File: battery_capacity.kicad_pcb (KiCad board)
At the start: 2 copper layers, 47 x 45 mm, 17 parts, among them J1 Screw_Terminal_01x03, J2 Screw_Terminal_01x04, Q1 IRLML2060, Q2 IRLML2060, U1 PC817, U2 PC817, U3 YAAJ_DCDC_StepDown_LM2596

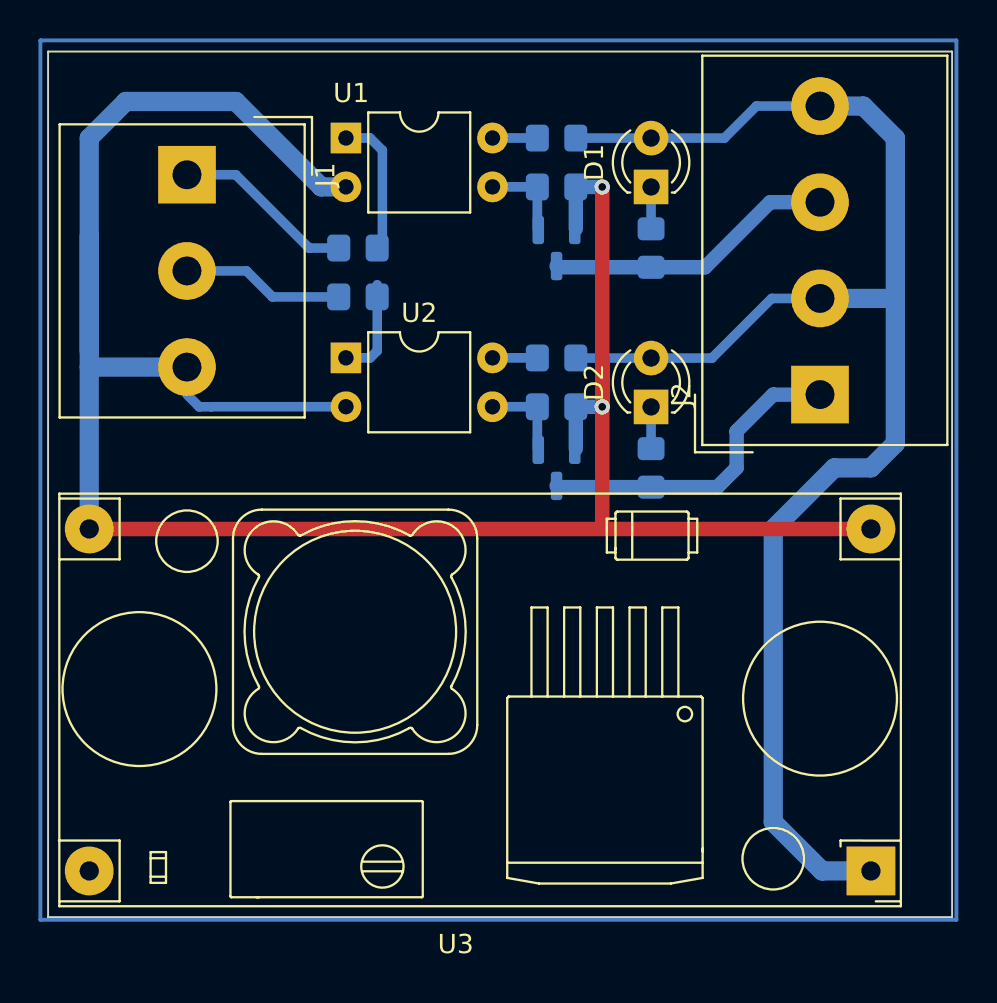
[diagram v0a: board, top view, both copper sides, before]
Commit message: h
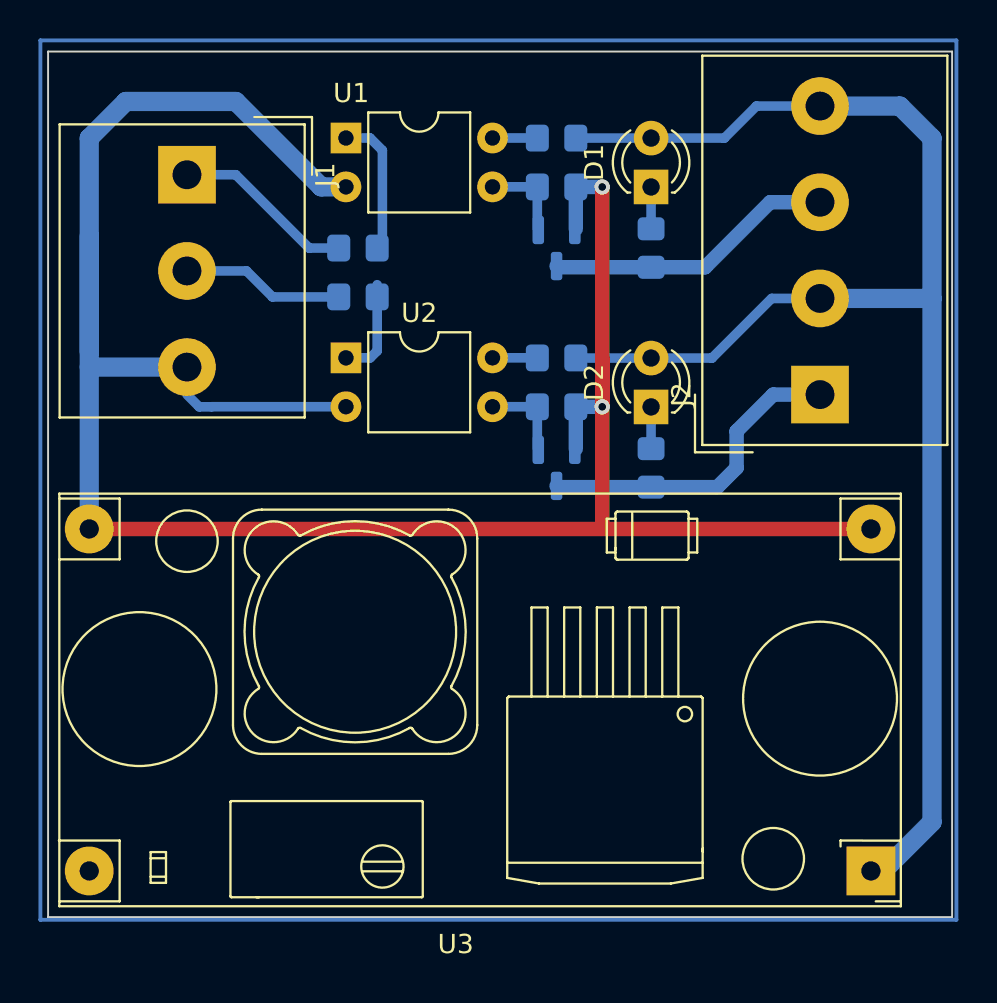
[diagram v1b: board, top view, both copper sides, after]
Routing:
- net +24V: track 81.4 -> 79.5 mm
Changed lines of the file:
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@@
     (fp_arc (start 9.481636 16.283217) (mid 9.510921 16.212508) (end 9.581636 16.183217)
       (stroke (width 0.12) (type solid)) (layer "F.SilkS"))
-    (fp_arc (start 9.581636 18.683217) (mid 9.510896 18.653941) (end 9.481636 18.583217)
-      (stroke (width 0.12) (type solid)) (layer "F.SilkS"))
-    (fp_arc (start 13.181636 16.183217) (mid 13.252317 16.21252) (end 13.281636 16.283217)
+    (fp_arc (start 9.581636 18.683217) (mid 9.510931 18.653935) (end 9.481636 18.583217)
+      (stroke (width 0.12) (type solid)) (layer "F.SilkS"))
+    (fp_arc (start 13.181636 16.183217) (mid 13.252353 16.212514) (end 13.281636 16.283217)
       (stroke (width 0.12) (type solid)) (layer "F.SilkS"))
     (fp_arc (start 13.281636 18.583217) (mid 13.252343 18.653929) (end 13.181636 18.683217)
@@
     (fp_arc (start 23.847611 17.472062) (mid 21.514153 17.739048) (end 21.781132 15.405582)
       (stroke (width 0.12) (type solid)) (layer "F.SilkS"))
-    (fp_arc (start 23.847611 17.472062) (mid 23.907831 17.428018) (end 23.981783 17.437976)
+    (fp_arc (start 23.847611 17.472062) (mid 23.907835 17.428062) (end 23.981783 17.437976)
       (stroke (width 0.12) (type solid)) (layer "F.SilkS"))
     (fp_arc (start 23.981783 7.433617) (mid 23.907854 7.443509) (end 23.847611 7.399531)
@@
     (stroke (width 0.1) (type default)) (fill none) (layer "Edge.Cuts"))
   (segment (start 133.35 68.215) (end 133.35 66.04) (width 0.5) (layer "B.Cu") (net 1))
-  (segment (start 146.05 63.5) (end 146.05 79.375) (width 1) (layer "B.Cu") (net 2))
-  (segment (start 146.05 79.375) (end 144.78 80.645) (width 1) (layer "B.Cu") (net 2))
-  (segment (start 145.97 71.835) (end 142.1325 71.835) (width 1) (layer "B.Cu") (net 2))
-  (segment (start 139.7 99.06) (end 142.24 101.6) (width 1) (layer "B.Cu") (net 2))
   (segment (start 129.435 74.93) (end 129.44 74.935) (width 0.25) (layer "B.Cu") (net 2))
   (segment (start 137.16 63.5) (end 133.35 63.5) (width 0.5) (layer "B.Cu") (net 2))
+  (segment (start 142.1325 61.835) (end 146.29 61.835) (width 1) (layer "B.Cu") (net 2))
   (segment (start 138.825 61.835) (end 137.16 63.5) (width 0.5) (layer "B.Cu") (net 2))
-  (segment (start 142.1325 61.835) (end 144.385 61.835) (width 1) (layer "B.Cu") (net 2))
-  (segment (start 142.24 101.6) (end 144.78 101.6) (width 1) (layer "B.Cu") (net 2))
-  (segment (start 144.385 61.835) (end 146.05 63.5) (width 1) (layer "B.Cu") (net 2))
+  (segment (start 145.415 101.6) (end 144.78 101.6) (width 1) (layer "B.Cu") (net 2))
+  (segment (start 147.955 71.835) (end 142.1325 71.835) (width 1) (layer "B.Cu") (net 2))
+  (segment (start 146.29 61.835) (end 147.955 63.5) (width 1) (layer "B.Cu") (net 2))
   (segment (start 133.35 74.935) (end 136.52 74.935) (width 0.5) (layer "B.Cu") (net 2))
   (segment (start 139.62 71.835) (end 142.1325 71.835) (width 0.5) (layer "B.Cu") (net 2))
   (segment (start 136.52 74.935) (end 139.62 71.835) (width 0.5) (layer "B.Cu") (net 2))
   (segment (start 129.435 63.5) (end 133.35 63.5) (width 0.5) (layer "B.Cu") (net 2))
-  (segment (start 146.05 71.755) (end 145.97 71.835) (width 1) (layer "B.Cu") (net 2))
-  (segment (start 144.78 80.645) (end 142.875 80.645) (width 1) (layer "B.Cu") (net 2))
-  (segment (start 142.875 80.645) (end 139.7 83.82) (width 1) (layer "B.Cu") (net 2))
+  (segment (start 147.955 99.06) (end 145.415 101.6) (width 1) (layer "B.Cu") (net 2))
   (segment (start 142.1325 61.835) (end 138.825 61.835) (width 0.5) (layer "B.Cu") (net 2))
-  (segment (start 139.7 83.82) (end 139.7 99.06) (width 1) (layer "B.Cu") (net 2))
+  (segment (start 147.955 63.5) (end 147.955 99.06) (width 1) (layer "B.Cu") (net 2))
   (segment (start 129.44 74.935) (end 133.35 74.935) (width 0.5) (layer "B.Cu") (net 2))
   (segment (start 133.35 79.645) (end 133.35 77.475) (width 0.5) (layer "B.Cu") (net 3))
